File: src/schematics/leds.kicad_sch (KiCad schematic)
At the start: 6 parts

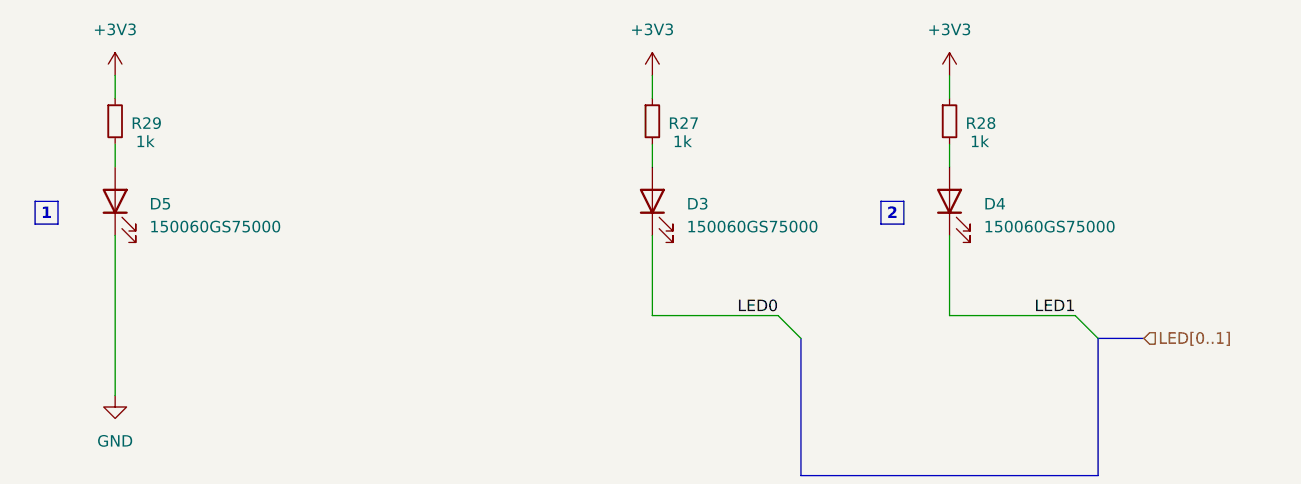
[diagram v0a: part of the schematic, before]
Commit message: Add bom components
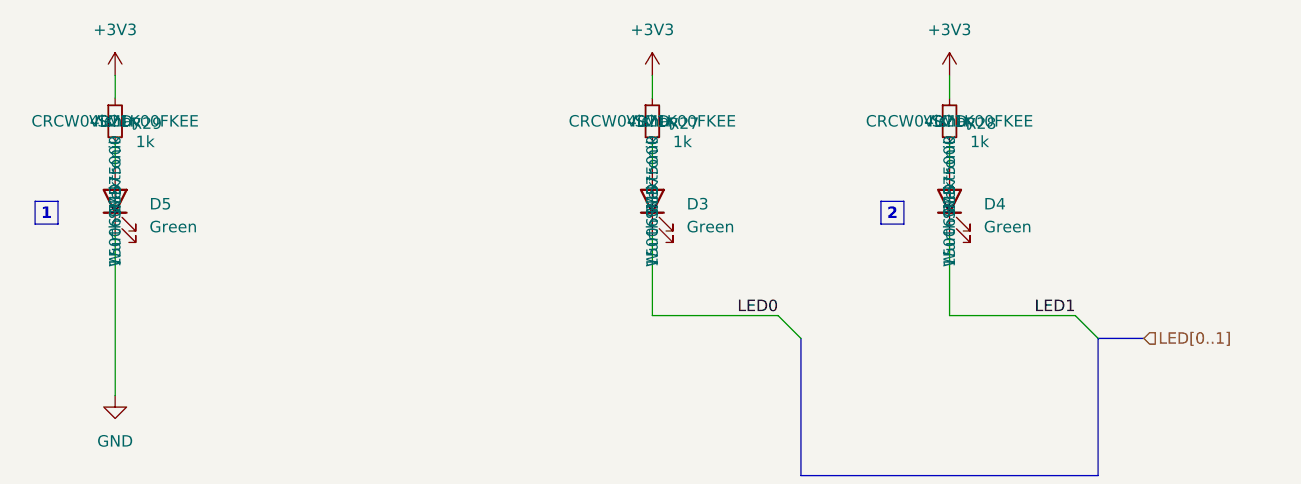
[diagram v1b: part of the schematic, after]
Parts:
- D3, D4, D5: value 150060GS75000 -> Green; MPN (none) -> 150060GS75000; Manufacturer (none) -> Wurth Elektronik; Mouting Technology (none) -> SMD
- R27, R28, R29: MPN (none) -> CRCW04021K00FKEE; Manufacturer (none) -> Vishay; Mouting Technology (none) -> SMD
